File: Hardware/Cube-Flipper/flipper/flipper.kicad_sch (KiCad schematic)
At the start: 2 parts, among them J1 Cube Orange Plus Male Header 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, J2 Cube Orange Plus Female Header

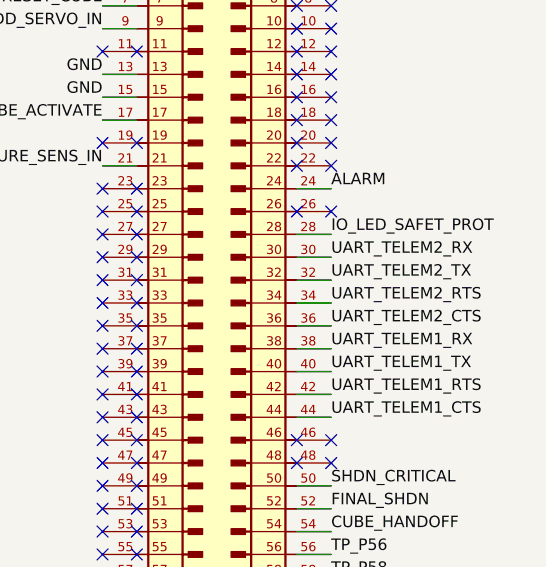
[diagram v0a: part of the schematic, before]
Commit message: complete flipper i really hope I didn't cook it
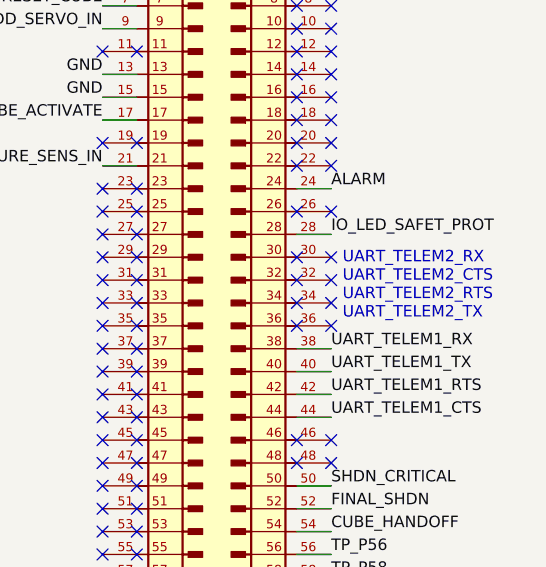
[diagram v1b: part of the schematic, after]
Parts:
- J1: footprint obad_footprints:CONN_DF173p0H-80DS-0p5V57_80P_HIR -> obad_footprints:Cube_Orange_Cube_Side
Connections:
- net UART_TELEM2_CTS: no longer names the net of J2.36
- net UART_TELEM2_CTS: no longer J1.36
- net UART_TELEM2_RTS: no longer names the net of J2.34
- net UART_TELEM2_RTS: no longer J1.34
- net UART_TELEM2_RX: no longer names the net of J2.30
- net UART_TELEM2_RX: no longer J1.30
- net UART_TELEM2_TX: no longer names the net of J2.32
- net UART_TELEM2_TX: no longer J1.32
- no-connect marks 92 -> 100
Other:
- note added: "UART_TELEM2_RX UART_TELEM2_CTS UART_TELEM2_RTS UART_TELEM2_TX"
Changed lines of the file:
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@@
 	(generator_version "9.0")
 	(paper "A4")
+	(text "UART_TELEM2_RX\nUART_TELEM2_CTS\nUART_TELEM2_RTS\nUART_TELEM2_TX"
+		(exclude_from_sim no)
+		(at 156.21 87.63 0)
+		(effects
+			(font
+				(size 1.27 1.27)
+			)
+			(justify left)
+		)
+	)
 	(no_connect
 		(at 133.35 92.075)
@@
 	)
 	(no_connect
+		(at 154.94 86.995)
+	)
+	(no_connect
+		(at 151.13 86.995)
+	)
+	(no_connect
 		(at 154.94 145.415)
 	)
@@
 	)
 	(no_connect
+		(at 154.94 84.455)
+	)
+	(no_connect
 		(at 151.13 107.315)
 	)
@@
 	)
 	(no_connect
+		(at 154.94 89.535)
+	)
+	(no_connect
+		(at 151.13 92.075)
+	)
+	(no_connect
 		(at 129.54 86.995)
 	)
@@
 	)
 	(no_connect
+		(at 151.13 84.455)
+	)
+	(no_connect
 		(at 154.94 132.715)
 	)
@@
 	)
 	(no_connect
+		(at 151.13 89.535)
+	)
+	(no_connect
 		(at 129.54 102.235)
 	)
@@
 	)
 	(no_connect
+		(at 154.94 92.075)
+	)
+	(no_connect
 		(at 129.54 114.935)
 	)
@@
 	(wire
 		(pts
-			(xy 151.13 89.535) (xy 154.94 89.535)
-		)
-		(stroke
-			(width 0)
-			(type default)
-		)
-	)
-	(wire
-		(pts
 			(xy 129.54 56.515) (xy 133.35 56.515)
 		)
@@
 	(wire
 		(pts
-			(xy 151.13 92.075) (xy 154.94 92.075)
-		)
-		(stroke
-			(width 0)
-			(type default)
-		)
-	)
-	(wire
-		(pts
-			(xy 151.13 86.995) (xy 154.94 86.995)
-		)
-		(stroke
-			(width 0)
-			(type default)
-		)
-	)
-	(wire
-		(pts
 			(xy 129.54 125.095) (xy 133.35 125.095)
 		)
@@
 		(pts
 			(xy 151.13 122.555) (xy 154.94 122.555)
-		)
-		(stroke
-			(width 0)
-			(type default)
-		)
-	)
-	(wire
-		(pts
-			(xy 151.13 84.455) (xy 154.94 84.455)
 		)
 		(stroke
@@
 		)
 	)
-	(label "UART_TELEM2_RX"
-		(at 154.94 84.455 0)
-		(effects
-			(font
-				(size 1.27 1.27)
-			)
-			(justify left bottom)
-		)
-	)
 	(label "CAN+"
 		(at 129.54 147.955 180)
@@
 		)
 	)
-	(label "UART_TELEM2_TX"
-		(at 154.94 86.995 0)
-		(effects
-			(font
-				(size 1.27 1.27)
-			)
-			(justify left bottom)
-		)
-	)
 	(label "TP_P56"
 		(at 154.94 117.475 0)
@@
 		)
 	)
-	(label "UART_TELEM2_CTS"
-		(at 154.94 92.075 0)
-		(effects
-			(font
-				(size 1.27 1.27)
-			)
-			(justify left bottom)
-		)
-	)
 	(label "VDD_SERVO_IN"
 		(at 129.54 59.055 180)
@@
 			)
 			(justify right bottom)
-		)
-	)
-	(label "UART_TELEM2_RTS"
-		(at 154.94 89.535 0)
-		(effects
-			(font
-				(size 1.27 1.27)
-			)
-			(justify left bottom)
 		)
 	)
@@
 			)
 		)
-		(property "Footprint" "obad_footprints:CONN_DF173p0H-80DS-0p5V57_80P_HIR"
+		(property "Footprint" "obad_footprints:Cube_Orange_Cube_Side"
 			(at 142.24 99.695 0)
 			(effects
